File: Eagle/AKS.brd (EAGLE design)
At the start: 100 x 54 mm, 13 parts, among them IC1 2982-DRV8825, IC2 2982-DRV8825

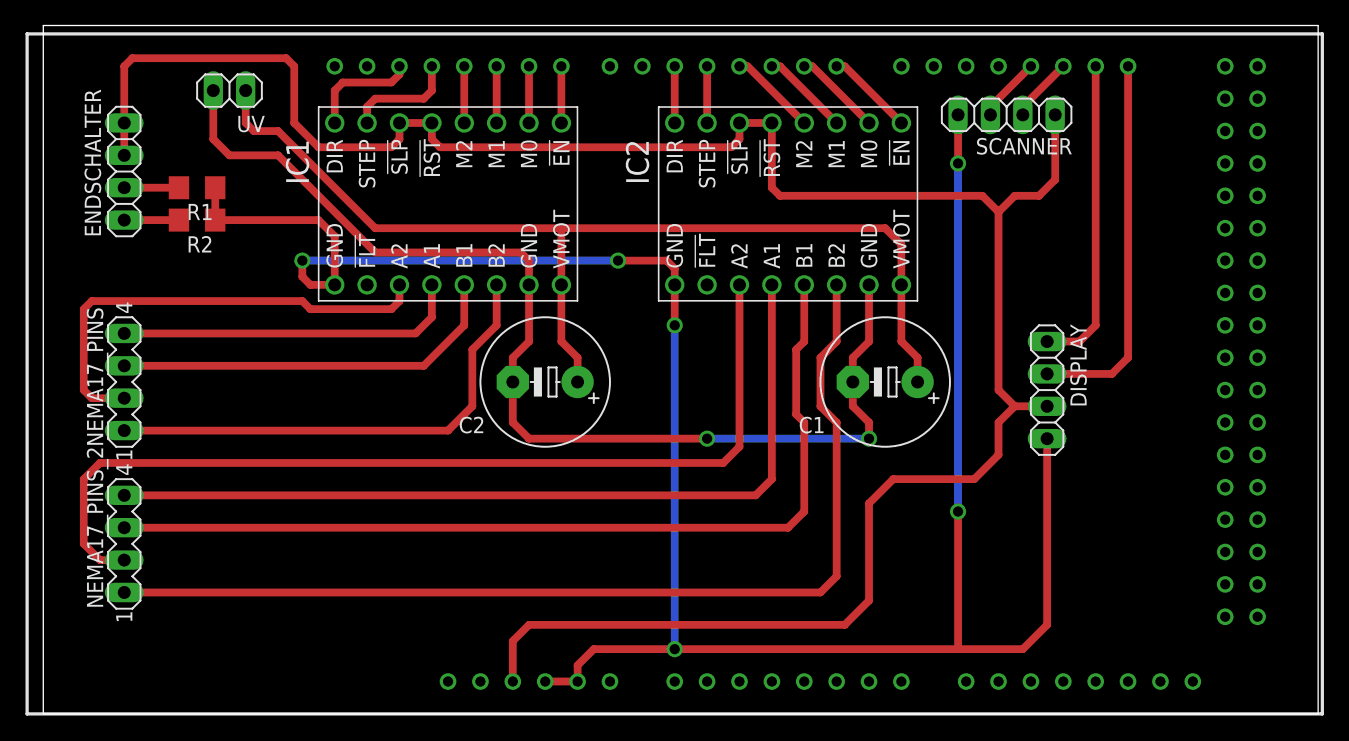
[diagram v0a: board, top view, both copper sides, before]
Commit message: hmmmm
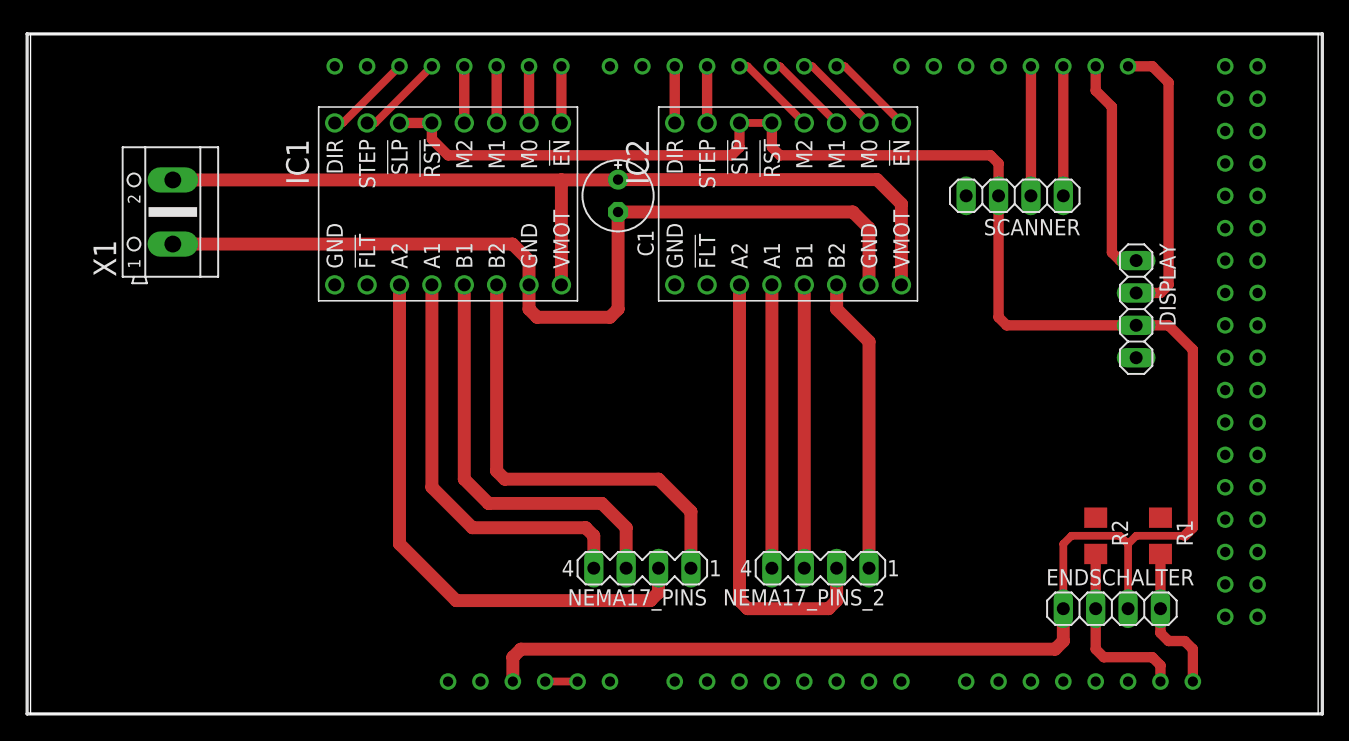
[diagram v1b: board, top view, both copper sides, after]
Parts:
- removed C2: 100uF, rcl:E5-10,5
- removed UV: (no value), HTL22_kontakte:1X02
- added X1: (no value), con-ptr500:AK500/2
- C1: value 100uF -> (none); device rcl:E5-10,5 -> rcl:E2,5-6E
- moved ENDSCHALTER 84.7 mm to (83.8, 8.26), turned to 0 degrees
- moved R1 80.3 mm to (87.6, 14.0), turned to 270 degrees
- moved R2 74.7 mm to (82.5, 14.0), turned to 270 degrees
- moved NEMA17_PINS_2 54.6 mm to (61.0, 11.4), turned to 180 degrees
- moved NEMA17_PINS 43.2 mm to (47.0, 11.4), turned to 180 degrees
- moved C1 25.5 mm to (45.1, 40.6), turned to 270 degrees
- moved DISPLAY 9.44 mm to (85.7, 31.8)
- moved SCANNER 6.38 mm to (76.2, 40.6)
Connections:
- removed net +40V: C1.+, C2.+, IC1.16, IC2.16, UV.1
- removed net N$9: ENDSCHALTER.2, R1.2
- new net +25V: C1.+, IC1.16, IC2.16, X1.2
- new net N$17: ENDSCHALTER.4, R1.2, U$3.A15
- net GND: now also U$3.GND@1
- net GND2: now also X1.1; no longer C2.-, UV.2
- net N$15: now also SCANNER.1; no longer SCANNER.2
- net N$16: now also SCANNER.2; no longer SCANNER.3
- net N$8: now also ENDSCHALTER.2, U$3.A14; no longer ENDSCHALTER.1
- net VCC: now also ENDSCHALTER.1, SCANNER.3; no longer ENDSCHALTER.4, SCANNER.1
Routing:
- net GND: track 178.1 -> 2.54 mm, vias 6 -> 0
- net +40V: track 81.8 -> 0.00 mm
- net +25V: track 0.00 -> 72.5 mm
- net N$4: track 80.3 -> 23.3 mm
- net N$5: track 72.2 -> 22.2 mm
- net N$6: track 66.6 -> 22.2 mm
- net N$7: track 74.0 -> 35.5 mm
- net GND2: track 87.3 -> 72.1 mm, vias 2 -> 0
- net N$17: track 0.00 -> 11.8 mm
- net VCC: track 176.8 -> 165.2 mm
- net N$8: track 4.29 -> 14.3 mm
- net N$10: track 36.6 -> 44.6 mm
- net N$13: track 24.7 -> 17.3 mm
- net N$14: track 29.7 -> 22.4 mm
- net N$3: track 27.2 -> 32.7 mm
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- added copper zone on layer 1, net GND
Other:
- board size 100 x 54 mm -> 101 x 53.3 mm
